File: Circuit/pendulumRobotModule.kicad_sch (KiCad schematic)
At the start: 28 parts, among them J1 Conn_01x02_Female, J2 conn_3x4, J3 Conn_01x02_Male, J4 Conn_01x04_Female, J5 conn_3x3, J6 Conn_01x02_Male, J7 Conn_01x04_Female, U1 ESP32-devKit, U2 MPU6050-breakout, U3 buckConverter-adj

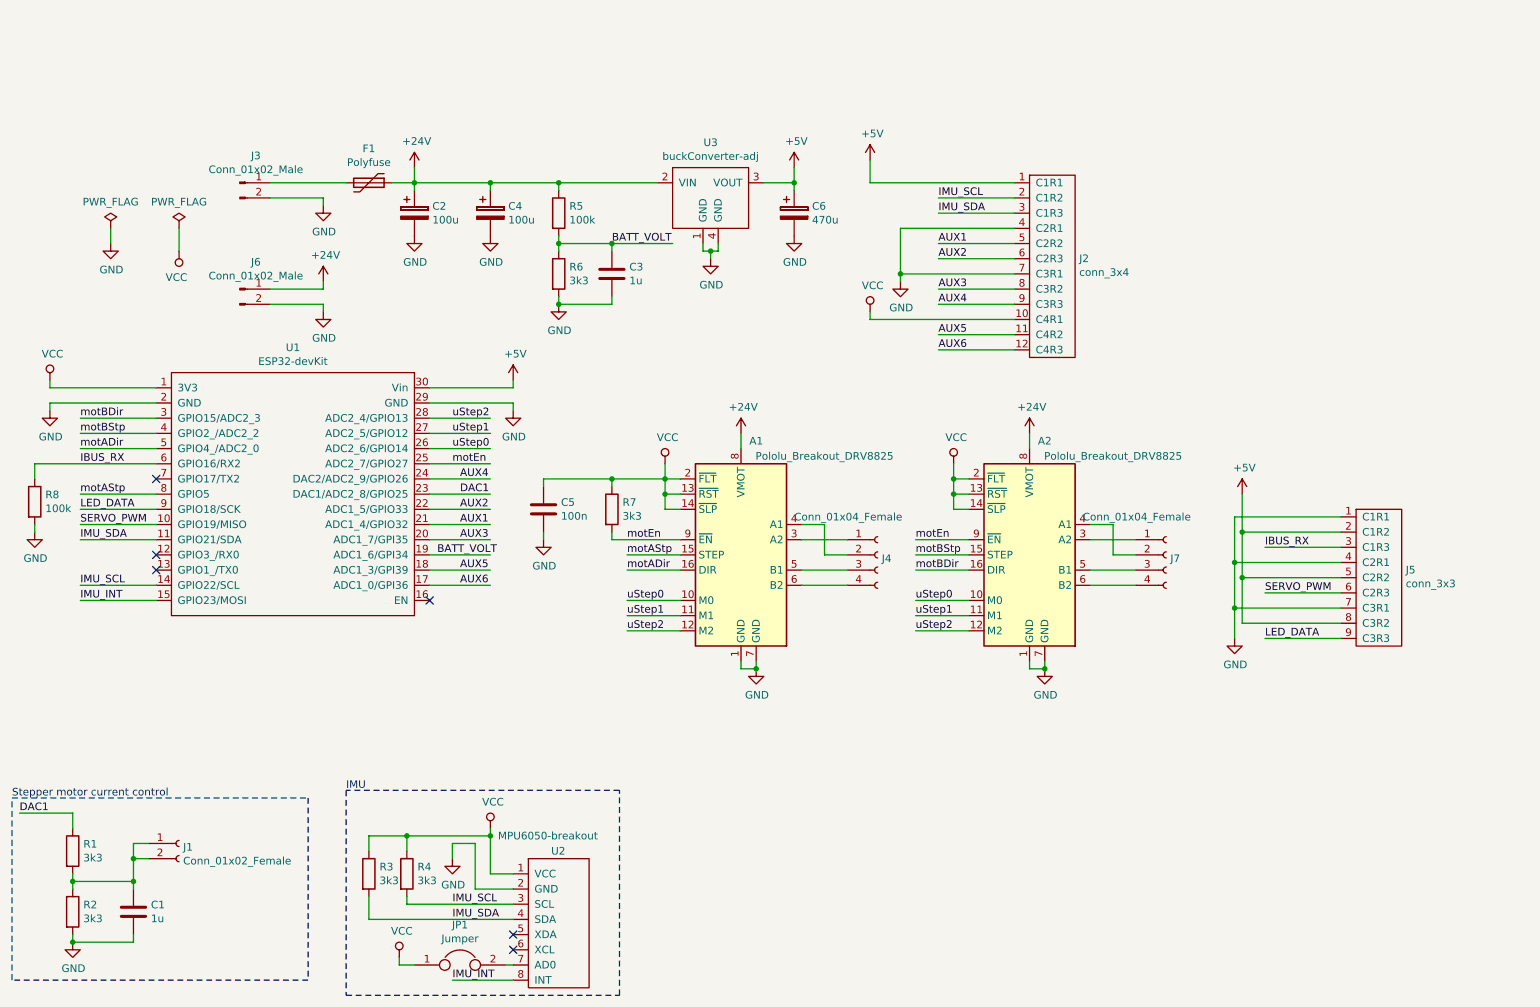
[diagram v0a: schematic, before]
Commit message: update
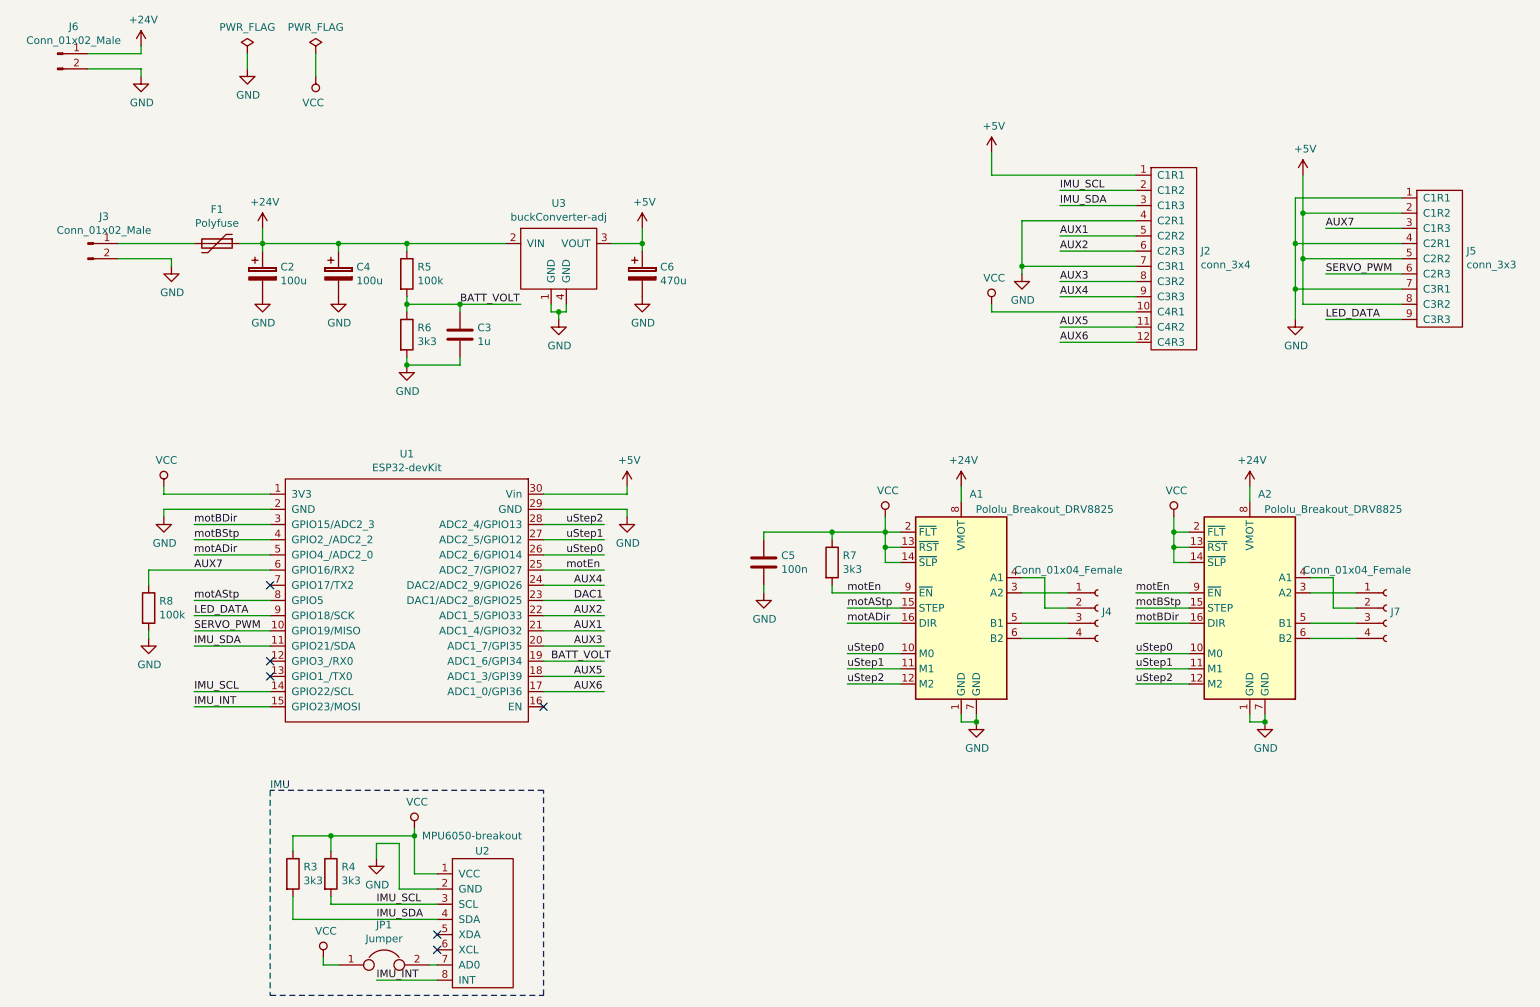
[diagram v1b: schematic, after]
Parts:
- removed C1: 1u, Capacitors_SMD:C_0805_HandSoldering, symbol Device:C
- removed J1: Conn_01x02_Female, Socket_Strips:Socket_Strip_Straight_1x02_Pitch2.54mm, symbol pendulumRobotModule-rescue:Conn_01x02_Female-Connector
- removed R1, R2: 3k3, Resistors_SMD:R_0805_HandSoldering, symbol Device:R
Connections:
- net IBUS_RX renamed AUX7
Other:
- note removed: "Stepper motor current control"
- company: (none) -> Digital Systems Project
- title: (none) -> Self Balncing Robot
- moved on the sheet: A1, A2, C2, C3, C4, C5, C6, F1, J2, J3, J4, J5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
